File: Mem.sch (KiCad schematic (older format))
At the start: 9 parts, among them U10 74AHC245, U2 74AHC245, U3 SRAM-512Kx16-TSOP2-44, U4 SRAM-512Kx16-TSOP2-44, U5 SRAM-512Kx16-TSOP2-44, U6 74AHC245, U7 74AHC245, U8 SRAM-512Kx16-TSOP2-44, U9 74AHC245

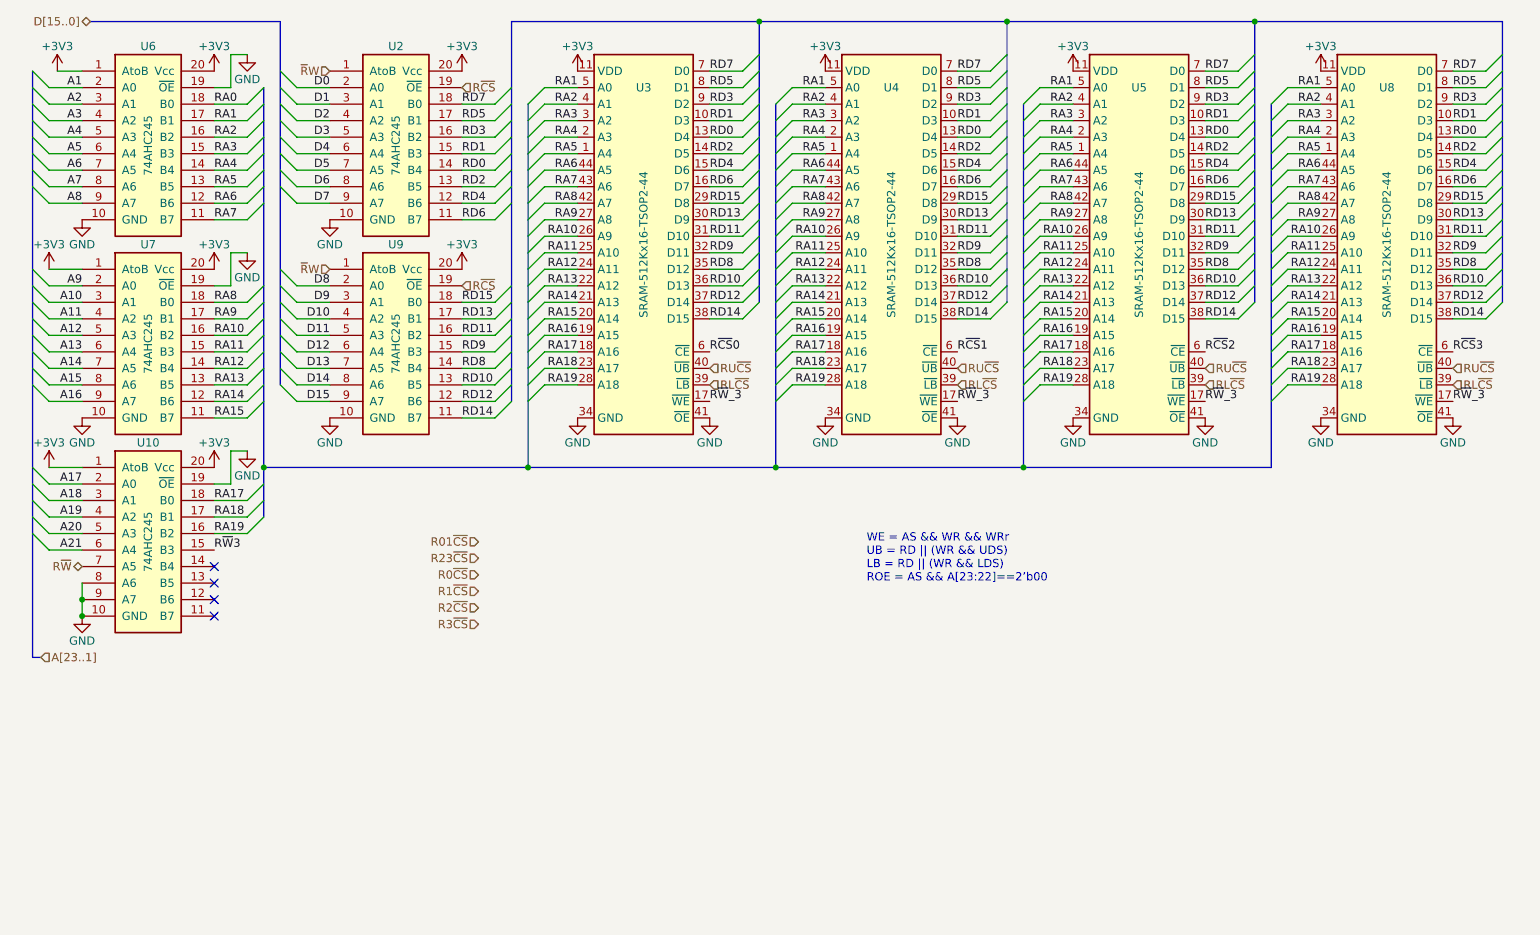
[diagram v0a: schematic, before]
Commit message: idk
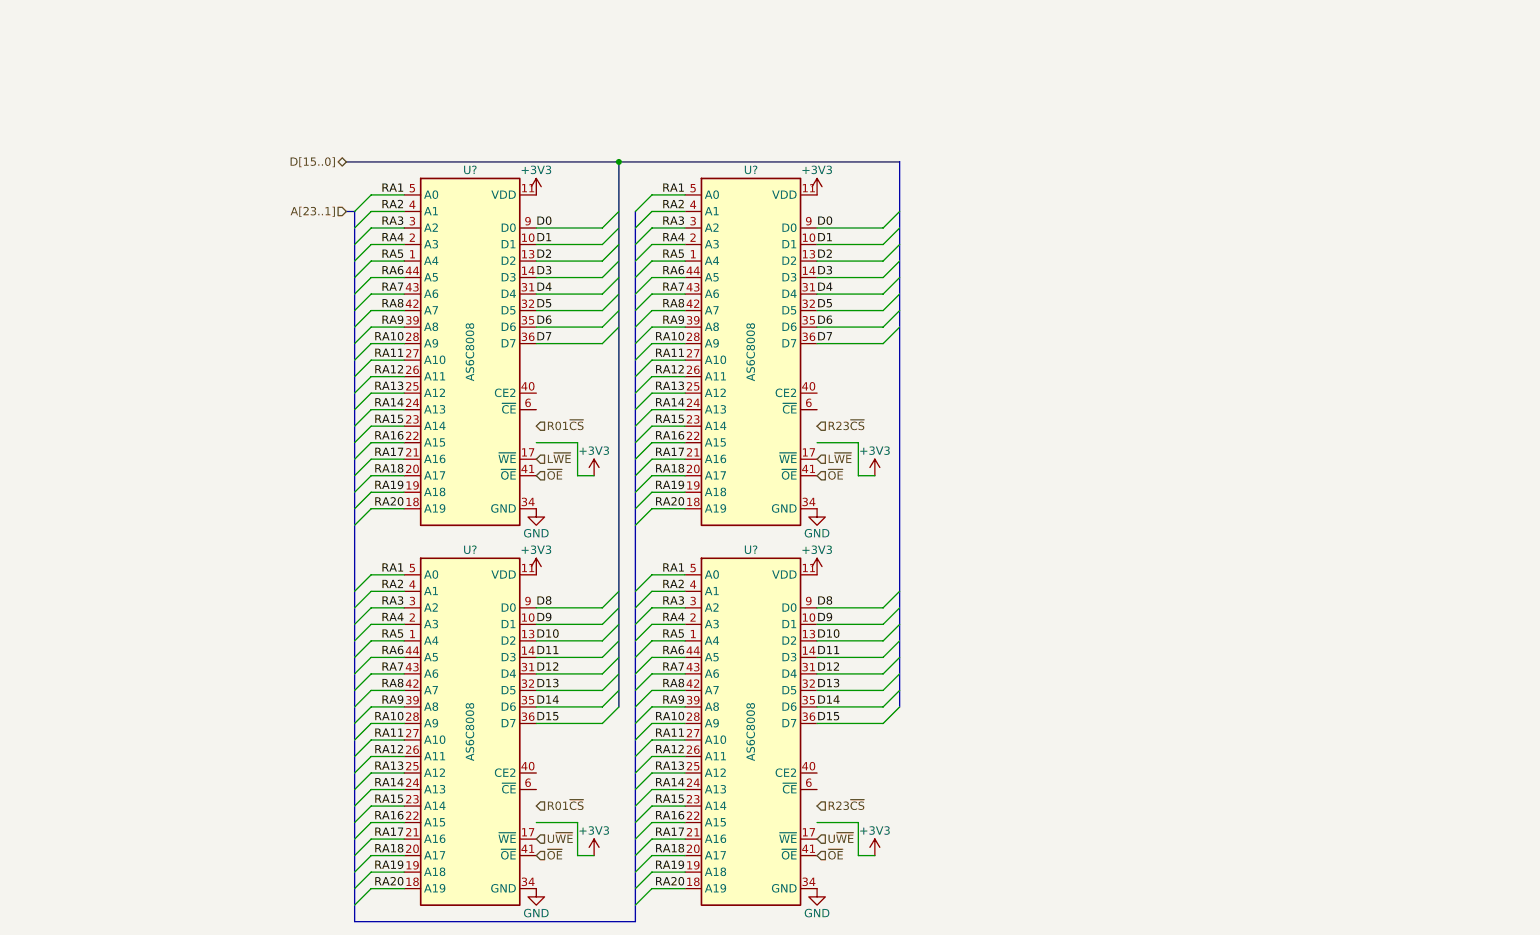
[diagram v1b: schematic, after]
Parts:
- removed U10, U2, U6, U7, U9: 74AHC245, stdpads:TSSOP-20_4.4x6.5mm_P0.65mm, symbol GW_Logic:74245
- removed U3, U4, U5, U8: SRAM-512Kx16-TSOP2-44, stdpads:TSOP-II-44_400mil_P0.8mm, symbol GW_RAM:SRAM-512Kx16-TSOP2-44
- added U? (x4): AS6C8008, stdpads:TSOP-II-44_400mil_P0.8mm, symbol GW_RAM:SRAM-1Mx8-TSOP2-44
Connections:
- net +3V3: now also U?.11 (VDD), U?.11 (VDD), U?.11 (VDD), U?.11 (VDD), U?.33 (VDD), U?.33 (VDD), U?.33 (VDD), U?.33 (VDD)
- net D0: now also U?.9 (D0), U?.9 (D0)
- net D1: now also U?.10 (D1), U?.10 (D1)
- net D10: now also U?.13 (D2), U?.13 (D2)
- net D11: now also U?.14 (D3), U?.14 (D3)
- net D12: now also U?.31 (D4), U?.31 (D4)
- net D13: now also U?.32 (D5), U?.32 (D5)
- net D14: now also U?.35 (D6), U?.35 (D6)
- net D15: now also U?.36 (D7), U?.36 (D7)
- net D2: now also U?.13 (D2), U?.13 (D2)
- net D3: now also U?.14 (D3), U?.14 (D3)
- net D4: now also U?.31 (D4), U?.31 (D4)
- net D5: now also U?.32 (D5), U?.32 (D5)
- net D6: now also U?.35 (D6), U?.35 (D6)
- net D7: now also U?.36 (D7), U?.36 (D7)
- net D8: now also U?.9 (D0), U?.9 (D0)
- net D9: now also U?.10 (D1), U?.10 (D1)
- net GND: now also U?.12 (GND), U?.12 (GND), U?.12 (GND), U?.12 (GND), U?.34 (GND), U?.34 (GND), U?.34 (GND), U?.34 (GND)
- net RA1: now also U?.5 (A0), U?.5 (A0), U?.5 (A0), U?.5 (A0)
- net RA10: now also U?.28 (A9), U?.28 (A9), U?.28 (A9), U?.28 (A9)
- net RA11: now also U?.27 (A10), U?.27 (A10), U?.27 (A10), U?.27 (A10)
- net RA12: now also U?.26 (A11), U?.26 (A11), U?.26 (A11), U?.26 (A11)
- net RA13: now also U?.25 (A12), U?.25 (A12), U?.25 (A12), U?.25 (A12)
- net RA14: now also U?.24 (A13), U?.24 (A13), U?.24 (A13), U?.24 (A13)
- net RA15: now also U?.23 (A14), U?.23 (A14), U?.23 (A14), U?.23 (A14)
- net RA16: now also U?.22 (A15), U?.22 (A15), U?.22 (A15), U?.22 (A15)
- net RA17: now also U?.21 (A16), U?.21 (A16), U?.21 (A16), U?.21 (A16)
- net RA18: now also U?.20 (A17), U?.20 (A17), U?.20 (A17), U?.20 (A17)
- net RA19: now also U?.19 (A18), U?.19 (A18), U?.19 (A18), U?.19 (A18)
- net RA2: now also U?.4 (A1), U?.4 (A1), U?.4 (A1), U?.4 (A1)
- net RA3: now also U?.3 (A2), U?.3 (A2), U?.3 (A2), U?.3 (A2)
- net RA4: now also U?.2 (A3), U?.2 (A3), U?.2 (A3), U?.2 (A3)
- net RA5: now also U?.1 (A4), U?.1 (A4), U?.1 (A4), U?.1 (A4)
- net RA6: now also U?.44 (A5), U?.44 (A5), U?.44 (A5), U?.44 (A5)
- net RA7: now also U?.43 (A6), U?.43 (A6), U?.43 (A6), U?.43 (A6)
- net RA8: now also U?.42 (A7), U?.42 (A7), U?.42 (A7), U?.42 (A7)
- net RA9: now also U?.39 (A8), U?.39 (A8), U?.39 (A8), U?.39 (A8)
- new net L~WE~: U?.17 (~WE~), U?.17 (~WE~)
- new net RA20: U?.18 (A19), U?.18 (A19), U?.18 (A19), U?.18 (A19)
- new net U~WE~: U?.17 (~WE~), U?.17 (~WE~)
- new net ~OE~: U?.41 (~OE~), U?.41 (~OE~), U?.41 (~OE~), U?.41 (~OE~)
- no-connect marks 4 -> 0
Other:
- note removed: "WE = AS && WR && WRr\nUB = RD || (WR && UDS)\nLB = RD || (WR && LDS)\nROE = AS && A[23:22]==2’b00"
